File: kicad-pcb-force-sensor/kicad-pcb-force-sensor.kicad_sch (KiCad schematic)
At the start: 20 parts, among them J1 Power, J2 Digital/PWM, J3 Analog, J4 Digital/PWM, M1 Motor_Servo, U3 KY-040

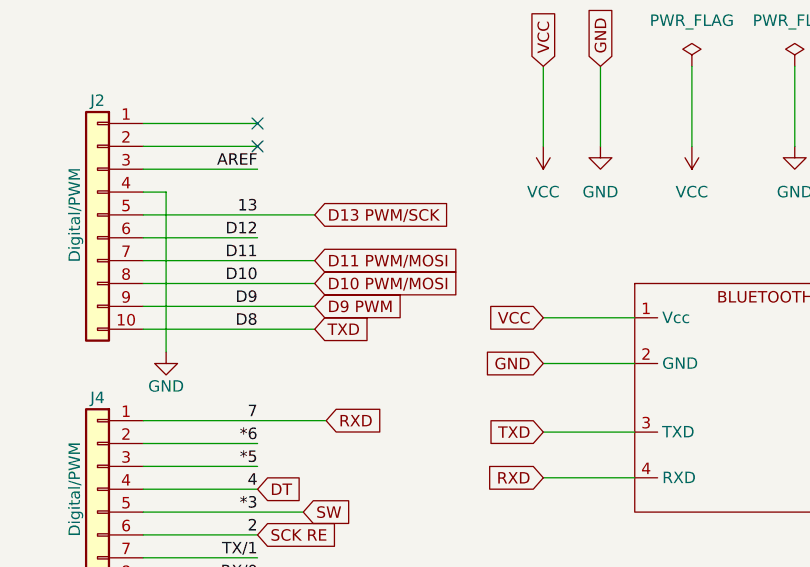
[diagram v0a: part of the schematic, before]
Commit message: Avec pistes
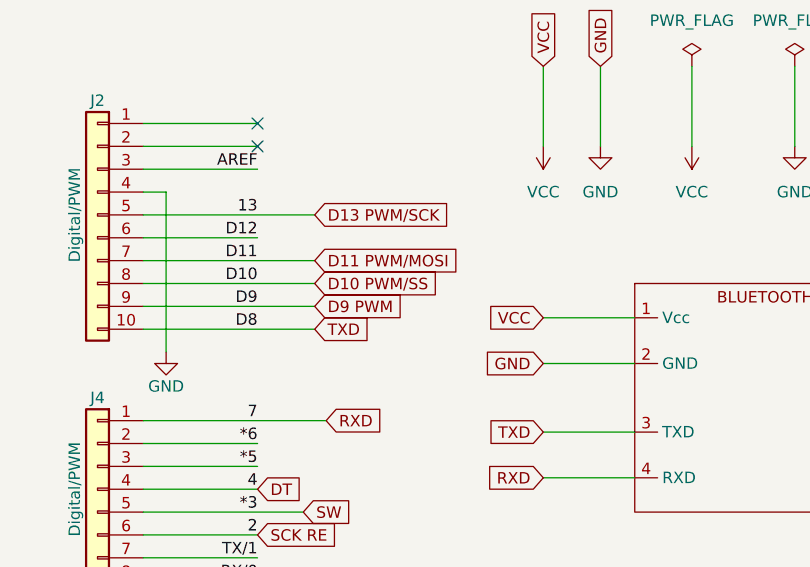
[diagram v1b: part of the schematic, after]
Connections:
- net D10 PWM/MOSI is gone; now on net D10 PWM/SS: J2.8 (Pin_8)
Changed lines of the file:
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@@
 		)
 	)
-	(global_label "D10 PWM{slash}MOSI"
+	(global_label "D10 PWM{slash}SS"
 		(shape input)
 		(at 81.28 44.45 0)
@@
 		)
 		(property "Intersheetrefs" "${INTERSHEET_REFS}"
-			(at 99.1164 44.45 0)
+			(at 96.9392 44.45 0)
 			(effects
 				(font
